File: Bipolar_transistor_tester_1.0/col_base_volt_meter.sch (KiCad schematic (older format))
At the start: 9 parts, among them Q1 PVG612, U3 CPC1977, U4 OP07

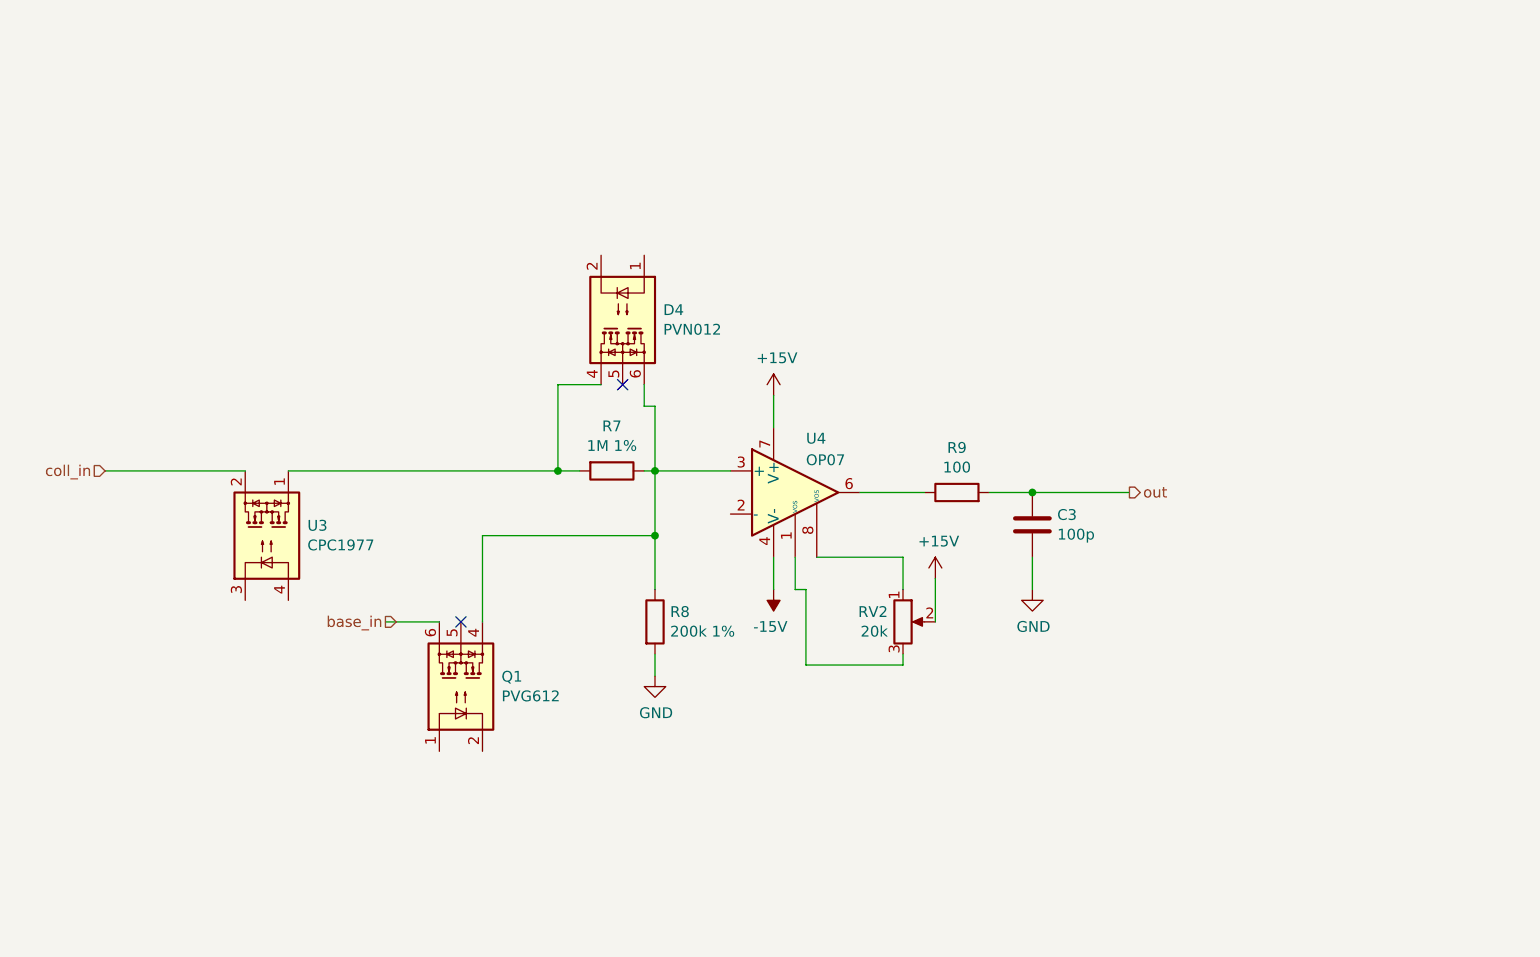
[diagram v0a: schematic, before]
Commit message: tester up
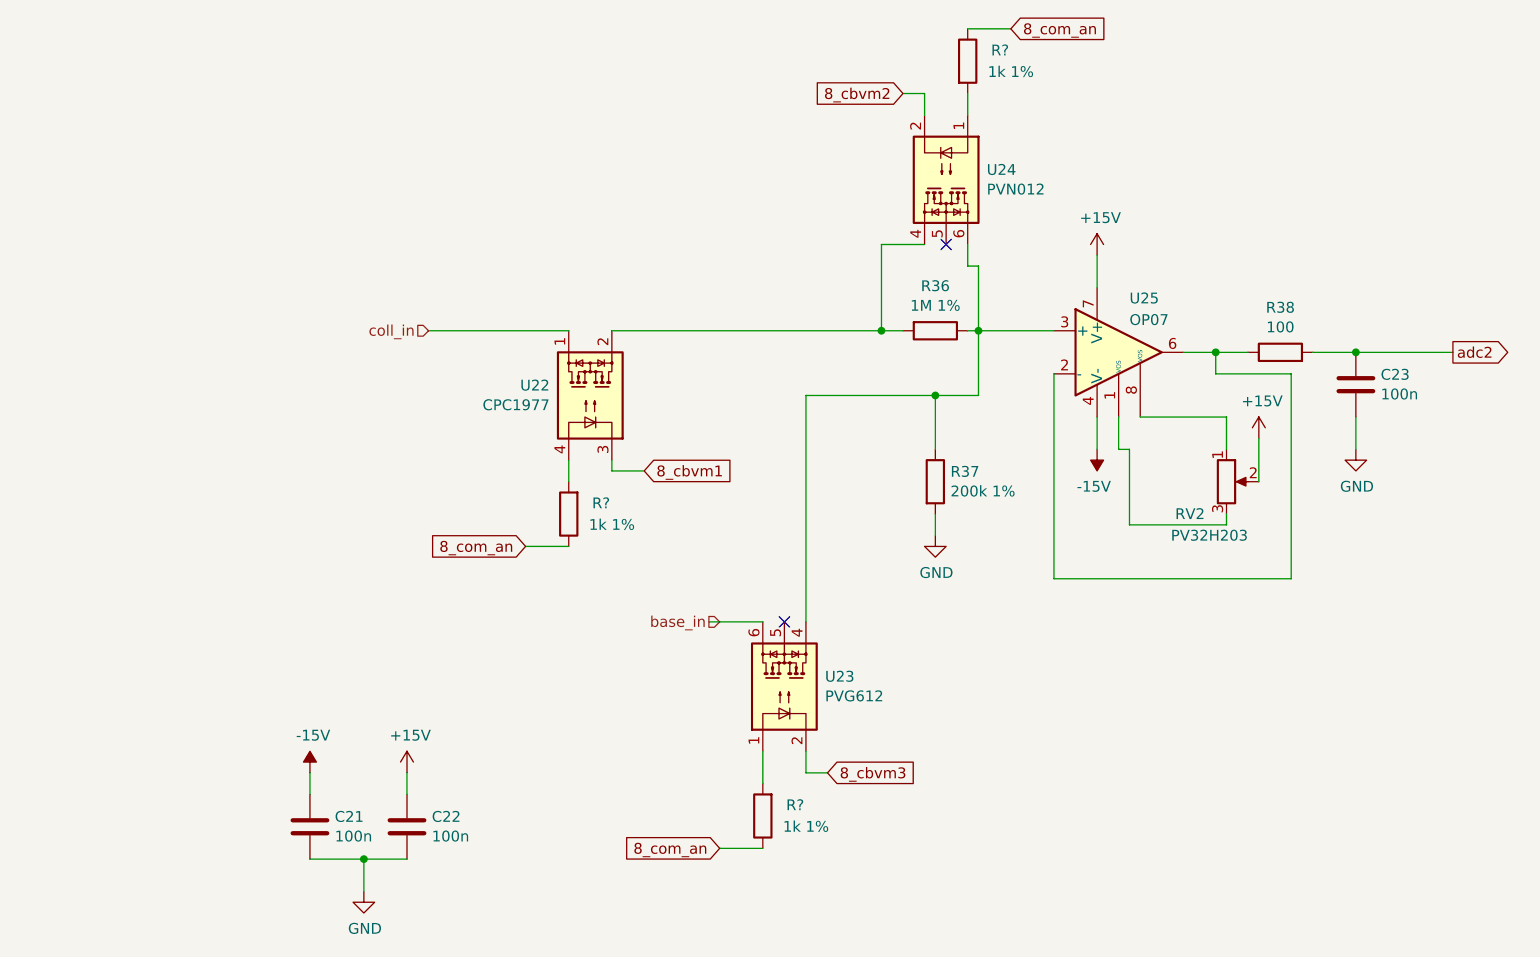
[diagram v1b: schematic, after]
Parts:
- added C21, C22: 100n, Capacitor_SMD:C_0805_2012Metric, symbol Device:C
- added R? (x3): 1k 1%, Resistor_SMD:R_0805_2012Metric, symbol Device:R
- C23: renamed from C3; value 100p -> 100n
- RV2: value 20k -> PV32H203; footprint (none) -> Potentiometer_THT:Potentiometer_Bourns_3339H_Vertical
- U22: renamed from U3; footprint (none) -> OptoDevice:i4-PAC
- U25: renamed from U4; footprint (none) -> Package_DIP:DIP-8_W7.62mm
- renumbered R7 to R36, R8 to R37, R9 to R38, Q1 to U23, D4 to U24
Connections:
- net labels added: 8_cbvm1, 8_cbvm2, 8_cbvm3, 8_com_an, adc2
- net labels removed: out
- wire segments 30 -> 54
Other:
- moved on the sheet: C23, R36, R37, R38, RV2, U22, U23, U24, U25
